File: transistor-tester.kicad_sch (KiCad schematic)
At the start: 23 parts, among them J1 Inputs, J2 PMOS Socket, J3 NMOS Socket, J4 PNP Socket, J5 NPN Socket, SW1 PMOS SW, SW2 NMOS SW, SW3 PNP SW, SW4 NPN SW

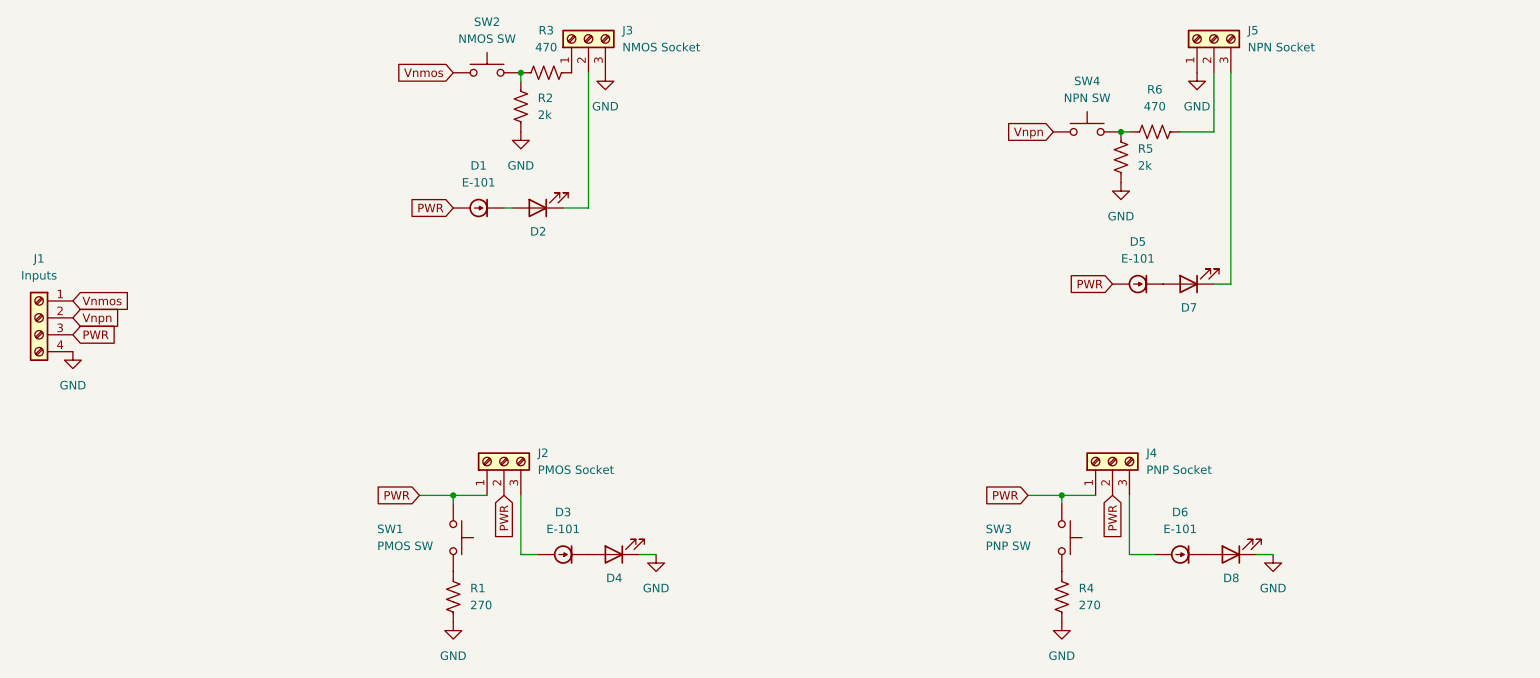
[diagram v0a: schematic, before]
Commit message: ?
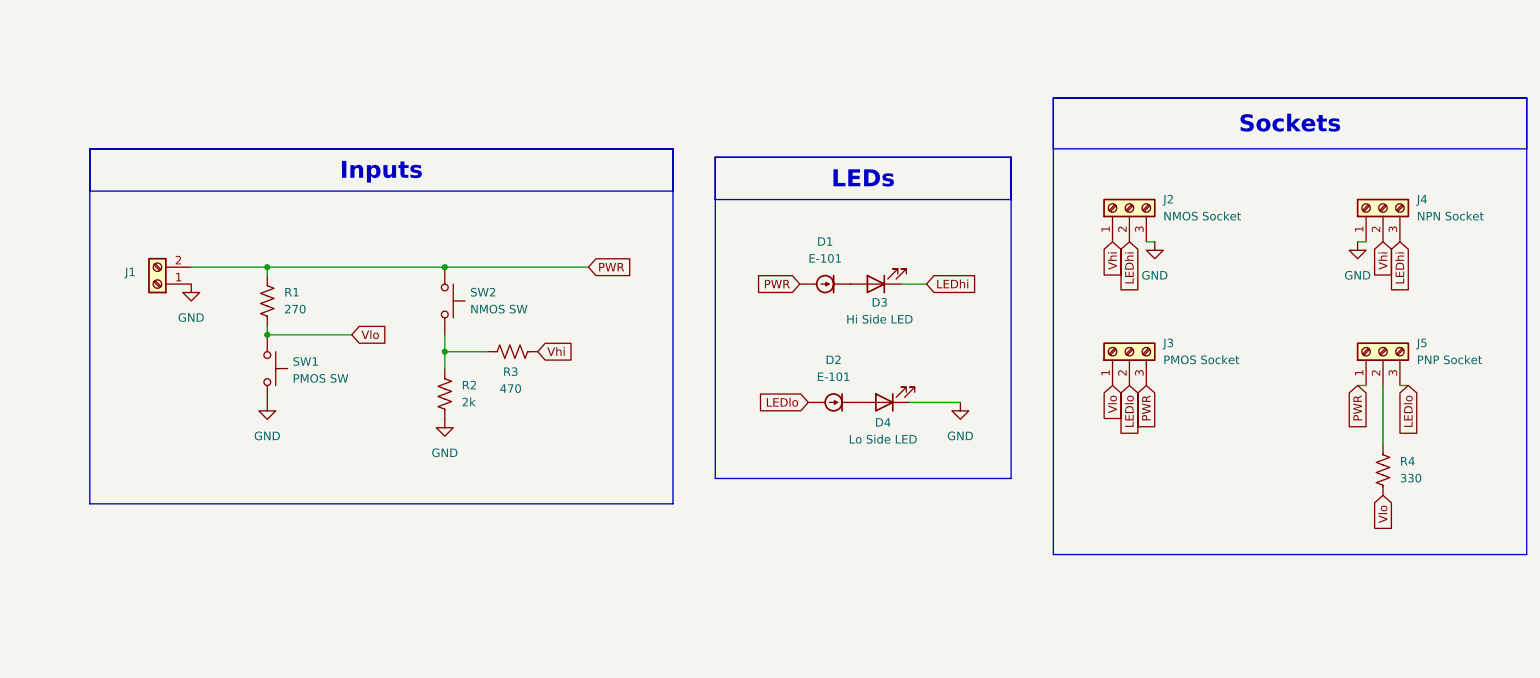
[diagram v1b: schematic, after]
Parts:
- removed D2, D8: NMOS LED, LED_THT:LED_D3.0mm_Clear, symbol Device:LED
- removed D3, D5, D6: E-101, symbol Device:D_Current-regulator
- removed D7: NPN LED, LED_THT:LED_D3.0mm_Clear, symbol Device:LED
- removed J1: Inputs, symbol Connector:Screw_Terminal_01x04
- removed R5: 2k, symbol Device:R_US
- removed R6: 470, symbol Device:R_US
- removed SW3: PNP SW, symbol Switch:SW_Push
- removed SW4: NPN SW, symbol Switch:SW_Push
- added D2: E-101, Diode_THT:D_A-405_P10.16mm_Horizontal, symbol Device:D_Current-regulator
- added D3: Hi Side LED, LED_THT:LED_D3.0mm, symbol Device:LED
- added J1: Screw_Terminal_01x02, TerminalBlock:TerminalBlock_MaiXu_MX126-5.0-02P_1x02_P5.00mm, symbol Connector:Screw_Terminal_01x02
- D1: footprint (none) -> Diode_THT:D_A-405_P10.16mm_Horizontal
- D4: value NMOS LED -> Lo Side LED; footprint LED_THT:LED_D3.0mm_Clear -> LED_THT:LED_D3.0mm
- R1, R2, R3: footprint (none) -> Resistor_THT:R_Axial_DIN0207_L6.3mm_D2.5mm_P10.16mm_Horizontal
- R4: value 270 -> 330; footprint (none) -> Resistor_THT:R_Axial_DIN0207_L6.3mm_D2.5mm_P10.16mm_Horizontal
- SW1, SW2: footprint (none) -> custom:Switch_PushButton_m12x0.75
- renumbered J3 to J2, J2 to J3, J5 to J4, J4 to J5
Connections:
- net Vnmos is gone; now on net PWR: SW2.1
- net GND: now also SW1.2, J1.1 (Pin_1); no longer R1.1, R4.1
- net PWR: now also J3.3 (Pin_3), R1.2, J1.2 (Pin_2); no longer J3.1 (Pin_1), J3.2 (Pin_2), J5.2 (Pin_2), SW1.1
- net at D1.1 (K): now also D3.2 (A)
- net at D4.2 (A): now also D2.1 (K)
- net Vhi: now reaches J2.1 (Pin_1), R3.2
- net Vhi: now also J4.2 (Pin_2)
- net LEDhi: now reaches J2.2 (Pin_2)
- net LEDhi: now also J4.3 (Pin_3), D3.1 (K)
- net LEDlo: now reaches J5.3 (Pin_3)
- net LEDlo: now also J3.2 (Pin_2), D2.2 (A)
- net Vlo: now reaches R4.2
- net Vlo: now also J3.1 (Pin_1), R1.1, SW1.1
- new net: J5.2 (Pin_2), R4.1
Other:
- moved on the sheet: D1, J2, J3, J4, J5
